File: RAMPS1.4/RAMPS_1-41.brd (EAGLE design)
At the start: 101.6 x 60.9 mm, 88 parts, among them Q1 STP55NF06L, Q2 STP55NF06L, Q3 STP55NF06L, U1 ARDUINO_MEGA_SHIELD, X4 MSTBA4

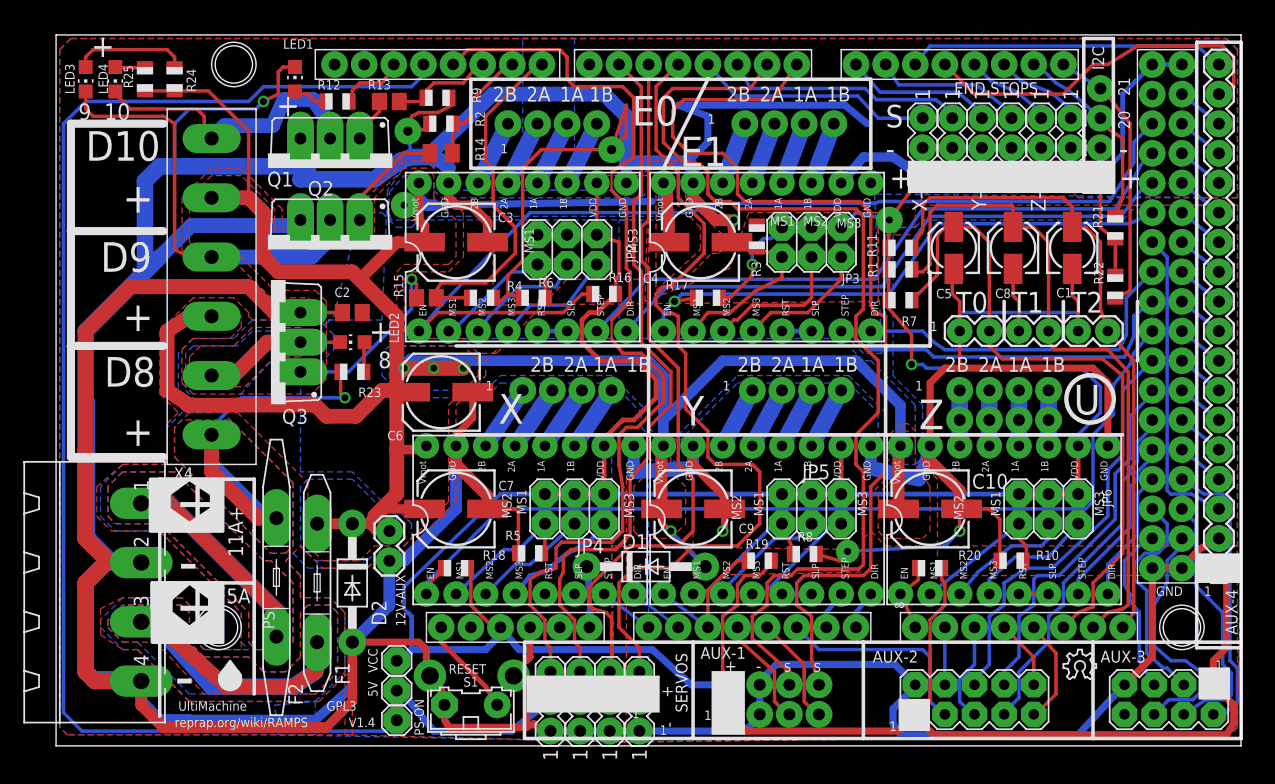
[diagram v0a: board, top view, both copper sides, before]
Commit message: add libs
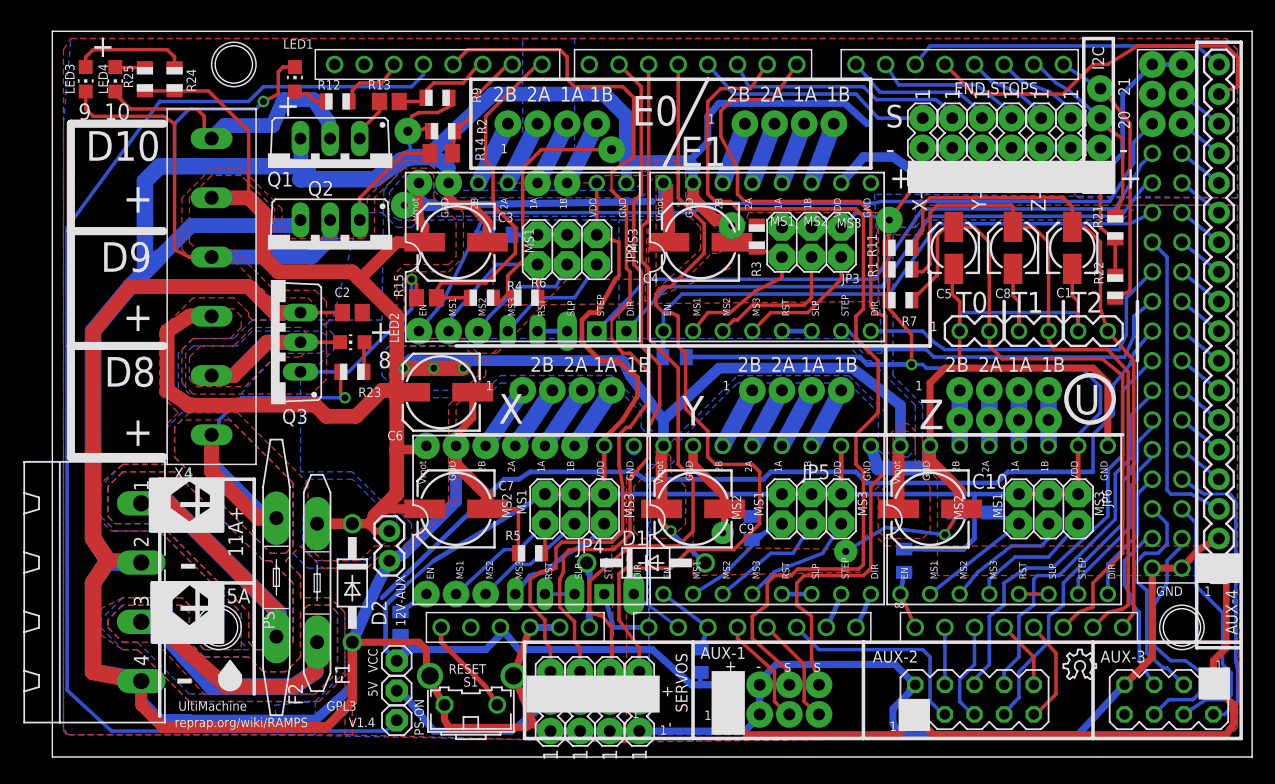
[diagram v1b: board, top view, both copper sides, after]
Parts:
- JP2, JP3, JP4, JP5, JP6: device pinhead:2X03 -> eagle-ramps:2X03
- R10: device adafruit:R0805 -> adafruit:R1206W
- U$4: device RepRapjr:A4988BREAKOUT -> e0:A4988BREAKOUT
- U$6: device RepRapjr:A4988BREAKOUT -> x:A4988BREAKOUT
- U1: device RepRapjr:ARDUINO_MEGA_SHIELD -> RepRapjr_o:ARDUINO_MEGA_SHIELD
- moved R16 10.2 mm to (38.1, 51.4), flipped to the bottom, turned to 0 degrees
- moved R19 9.96 mm to (55.2, 14.9), flipped to the bottom, turned to 90 degrees
- moved R18 6.74 mm to (29.5, 18.1), flipped to the bottom, turned to 90 degrees
- moved R17 5.83 mm to (53.0, 41.0), flipped to the bottom, turned to 0 degrees
- moved R10 5.21 mm to (78.7, 27.6), flipped to the bottom, turned to 0 degrees
- moved R8 5.08 mm to (59.6, 26.3), flipped to the bottom, turned to 90 degrees
- moved R20 2.31 mm to (72.7, 23.5), flipped to the bottom, turned to 270 degrees
- moved R2 0.65 mm to (33.2, 60.3)
- moved R6 0.64 mm to (40.3, 46.0)
- moved D1 0.32 mm to (50.6, 23.3)
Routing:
- net GND: track 668.0 -> 618.1 mm
- net E0-EN: track 87.9 -> 74.4 mm
- net VCC: track 352.8 -> 342.3 mm, vias 3 -> 2
- net D1: track 83.9 -> 76.2 mm
- net D2: track 86.5 -> 80.3 mm
- net D12: track 113.6 -> 107.5 mm
- net Y-EN: track 12.4 -> 6.73 mm
- net X-EN: track 81.0 -> 84.7 mm
- net +12V: track 230.1 -> 227.4 mm
- net D11: track 82.4 -> 80.2 mm
- net D4: track 72.5 -> 71.2 mm
- net X-STEP: track 4.76 -> 5.98 mm
- net Z-EN: track 6.09 -> 5.01 mm
- net N$40: track 13.3 -> 12.2 mm
- net D6: track 61.2 -> 60.3 mm
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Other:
- board size 101.6 x 60.9 mm -> 102.9 x 62.2 mm
